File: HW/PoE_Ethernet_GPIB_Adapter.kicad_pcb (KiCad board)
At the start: 6 copper layers, 60 x 55 mm, 198 parts, among them J1 ARJM11C7-114-BA-EW2, J2 112-024-113R001, J3 USB4105-GF-A, J4 UPDI Debug Connector, Q1 PMV30XPEAR, Q2 BC857BS, SW1 Reset, U1 LM5180, U10 AZ1117-3.3_SOT89, U11 TPS2375-1, U2 ATmega4809-A, U3 W5500, U4 24AA256UID, U5 USBLC6-2P6, U6 CH340X, U7 SN74LV1T125DCK, U8 SN74LV1T125DCK, U9 APX811-31UG-7, Y1 25Mhz

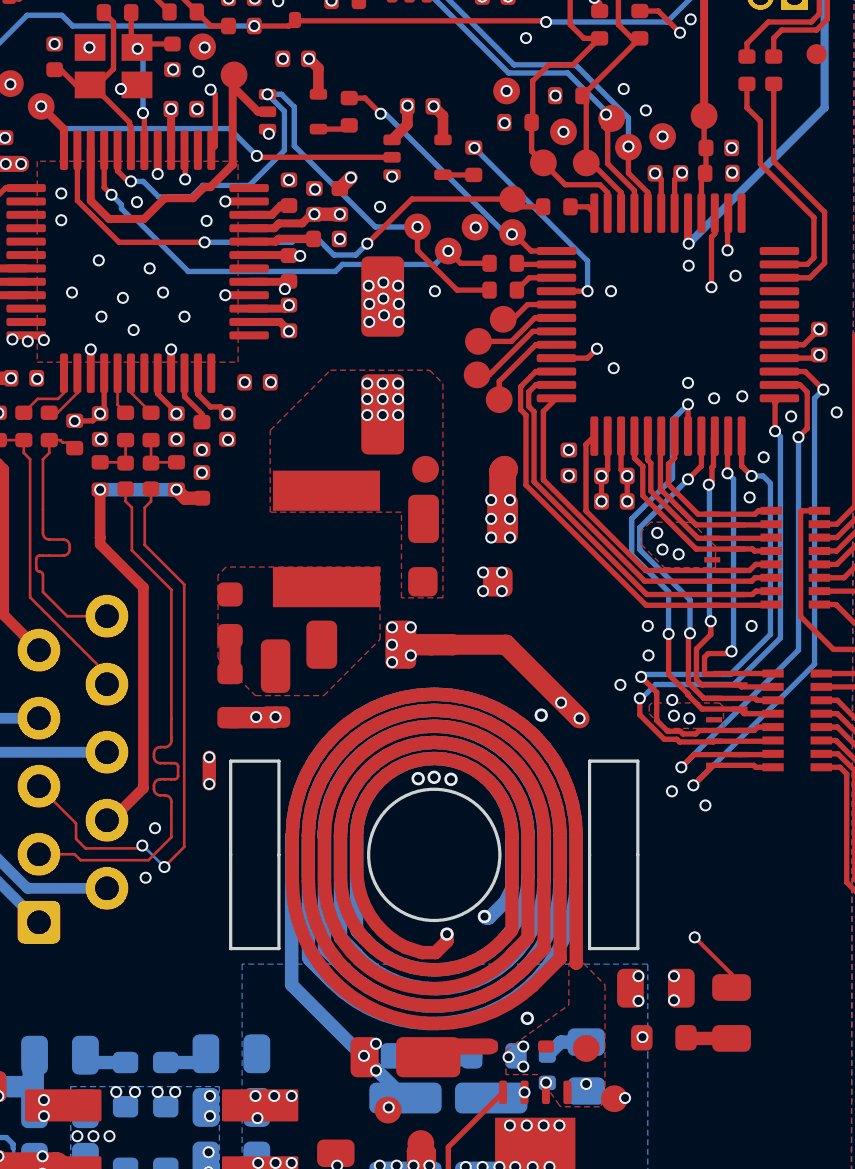
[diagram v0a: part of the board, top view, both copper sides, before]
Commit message: asdf
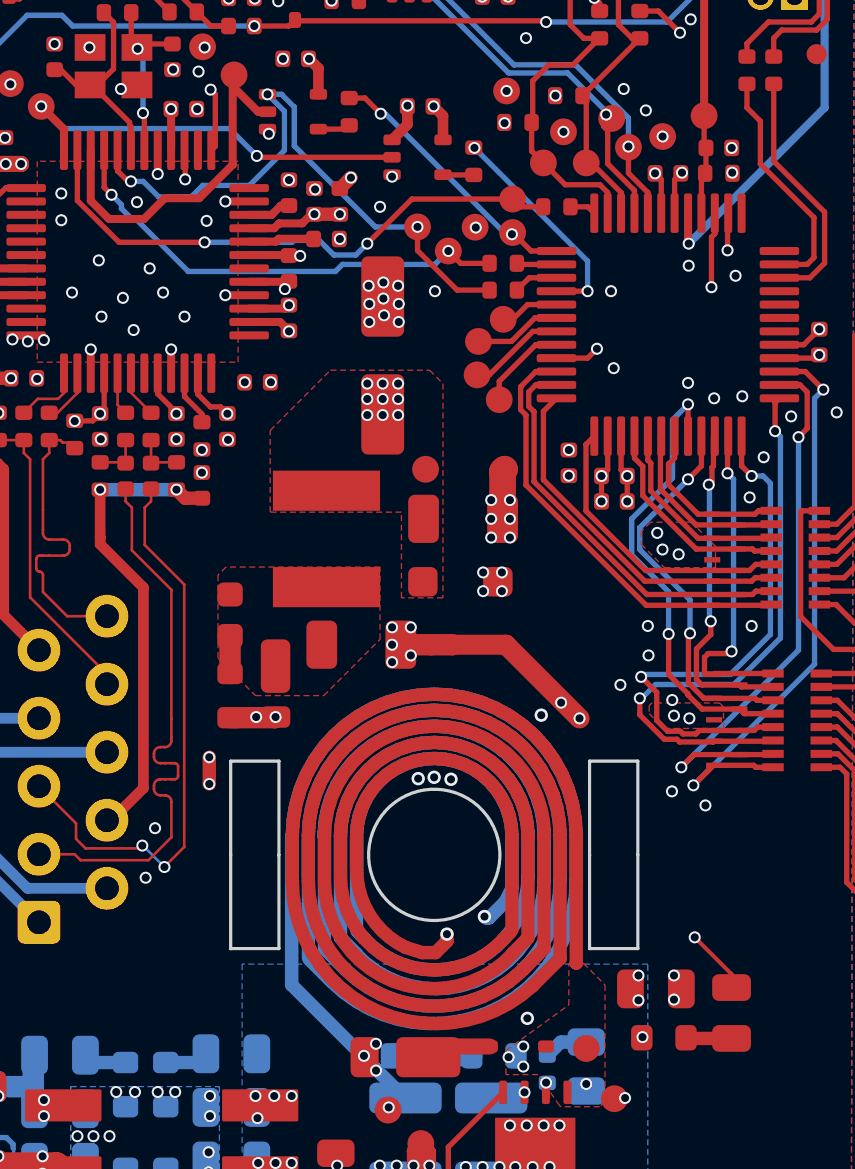
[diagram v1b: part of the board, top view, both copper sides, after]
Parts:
- turned C57 to 180 degrees
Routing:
- net Earth: track 6.68 -> 3.84 mm
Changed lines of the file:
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@@
 	(footprint "Capacitor_SMD:C_0805_2012Metric"
 		(layer "F.Cu")
-		(at 7.4 16.875)
+		(at 7.4 16.9 180)
 		(descr "Capacitor SMD 0805 (2012 Metric), square (rectangular) end terminal, IPC_7351 nominal, (Body size source: IPC-SM-782 page 76, https://www.pcb-3d.com/wordpress/wp-content/uploads/ipc-sm-782a_amendment_1_and_2.pdf, https://docs.google.com/spreadsheets/d/1BsfQQcO9C6DZCsRaXUlFlo91Tg2WpOkGARC1WS5S8t0/edit?usp=sharing), generated with kicad-footprint-generator")
 		(tags "capacitor")
 		(property "Reference" "C57"
-			(at 0 -1.68 0)
+			(at 0 -1.68 360)
 			(layer "User.1")
 			(effects
@@
 		)
 		(property "Value" "4.7n 1kV"
-			(at 0 1.68 0)
+			(at 0 1.68 360)
 			(layer "F.Fab")
 			(effects
@@
 		)
 		(property "Footprint" ""
-			(at 0 0 0)
+			(at 0 0 360)
 			(layer "F.Fab")
 			(hide yes)
@@
 		)
 		(property "Datasheet" ""
-			(at 0 0 0)
+			(at 0 0 180)
 			(unlocked yes)
 			(layer "F.Fab")
@@
 		)
 		(property "Description" "Unpolarized capacitor"
-			(at 0 0 0)
+			(at 0 0 180)
 			(unlocked yes)
 			(layer "F.Fab")
@@
 		)
 		(property "Model" "C0805C472KDRACTU"
-			(at 0 0 0)
+			(at 0 0 180)
 			(unlocked yes)
 			(layer "F.Fab")
@@
 		)
 		(property "Manufacturer" "KEMET"
-			(at 0 0 0)
+			(at 0 0 180)
 			(unlocked yes)
 			(layer "F.Fab")
@@
 		)
 		(property "JLCPCB" "C565695"
-			(at 0 0 0)
+			(at 0 0 180)
 			(unlocked yes)
 			(layer "F.Fab")
@@
 		(attr smd)
 		(fp_line
-			(start -1.7 -0.98)
-			(end 1.7 -0.98)
+			(start 1.7 0.98)
+			(end -1.7 0.98)
 			(stroke
 				(width 0.05)
@@
 		)
 		(fp_line
-			(start -1.7 0.98)
-			(end -1.7 -0.98)
+			(start 1.7 -0.98)
+			(end 1.7 0.98)
 			(stroke
 				(width 0.05)
@@
 		)
 		(fp_line
-			(start 1.7 -0.98)
-			(end 1.7 0.98)
+			(start -1.7 0.98)
+			(end -1.7 -0.98)
 			(stroke
 				(width 0.05)
@@
 		)
 		(fp_line
-			(start 1.7 0.98)
-			(end -1.7 0.98)
+			(start -1.7 -0.98)
+			(end 1.7 -0.98)
 			(stroke
 				(width 0.05)
@@
 		)
 		(fp_line
-			(start -1 -0.625)
-			(end 1 -0.625)
+			(start 1 0.625)
+			(end -1 0.625)
 			(stroke
 				(width 0.1)
@@
 		)
 		(fp_line
-			(start -1 0.625)
-			(end -1 -0.625)
+			(start 1 -0.625)
+			(end 1 0.625)
 			(stroke
 				(width 0.1)
@@
 		)
 		(fp_line
-			(start 1 -0.625)
-			(end 1 0.625)
+			(start -1 0.625)
+			(end -1 -0.625)
 			(stroke
 				(width 0.1)
@@
 		)
 		(fp_line
-			(start 1 0.625)
-			(end -1 0.625)
+			(start -1 -0.625)
+			(end 1 -0.625)
 			(stroke
 				(width 0.1)
@@
 		)
 		(fp_line
-			(start -0.261252 -0.735)
-			(end 0.261252 -0.735)
+			(start -0.261252 0.735)
+			(end 0.261252 0.735)
 			(stroke
 				(width 0.12)
@@
 		)
 		(fp_line
-			(start -0.261252 0.735)
-			(end 0.261252 0.735)
+			(start -0.261252 -0.735)
+			(end 0.261252 -0.735)
 			(stroke
 				(width 0.12)
@@
 		)
 		(fp_text user "${REFERENCE}"
-			(at 0 0 0)
+			(at 0 0 360)
 			(layer "F.Fab")
 			(effects
@@
 		)
 		(pad "1" smd roundrect
-			(at -0.95 0)
+			(at -0.95 0 180)
 			(size 1 1.45)
 			(layers "F.Cu" "F.Mask" "F.Paste")
@@
 		)
 		(pad "2" smd roundrect
-			(at 0.95 0)
+			(at 0.95 0 180)
 			(size 1 1.45)
 			(layers "F.Cu" "F.Mask" "F.Paste")
@@
 					(xy 2.562135 -23.67391) (xy 2.420116 -23.569076) (xy 2.256769 -23.480525) (xy 2.082437 -23.416511)
 					(xy 1.888964 -23.376857) (xy 1.67315 -23.363105) (xy 1.45746 -23.376857) (xy 1.26411 -23.416511)
-					(xy 1.089898 -23.480525) (xy 0.926442 -23.569094) (xy 0.78443 -23.673929) (xy 0.661803 -23.795415)
-					(xy 0.557004 -23.93306) (xy 0.469614 -24.086359) (xy 0.399486 -24.257034) (xy 0.331952 -24.526478)
-					(xy 0.309177 -24.810976) (xy 0.695325 -24.810976) (xy 0.711384 -24.579532) (xy 0.75834 -24.366027)
+					(xy 1.089898 -23.480525) (xy 0.926442 -23.569094) (xy 0.784429 -23.673929) (xy 0.661802 -23.795415)
+					(xy 0.557003 -23.93306) (xy 0.469613 -24.086359) (xy 0.399485 -24.257034) (xy 0.331951 -24.526478)
+					(xy 0.309176 -24.810976) (xy 0.695324 -24.810976) (xy 0.711383 -24.579532) (xy 0.758339 -24.366027)
 					(xy 0.837011 -24.168231) (xy 0.942986 -24.001128) (xy 1.079756 -23.862439) (xy 1.24945 -23.756397)
 					(xy 1.375374 -23.708186) (xy 1.515771 -23.6783) (xy 1.67315 -23.66792) (xy 1.830653 -23.6783) (xy 1.971173 -23.708186)
@@
 					(xy 2.097217 -25.863358) (xy 1.971056 -25.912802) (xy 1.830547 -25.94341) (xy 1.67315 -25.954033)
 					(xy 1.515877 -25.94341) (xy 1.375492 -25.912802) (xy 1.24945 -25.863358) (xy 1.079526 -25.756124)
-					(xy 0.942986 -25.618627) (xy 0.837114 -25.45336) (xy 0.75834 -25.255926) (xy 0.711384 -25.042421)
-					(xy 0.695325 -24.810976) (xy 0.309177 -24.810976) (xy 0.331952 -25.095475) (xy 0.399486 -25.364919)
-					(xy 0.469614 -25.535594) (xy 0.557004 -25.688893) (xy 0.661803 -25.826538) (xy 0.784436 -25.948009)
+					(xy 0.942986 -25.618627) (xy 0.837114 -25.45336) (xy 0.758339 -25.255926) (xy 0.711383 -25.042421)
+					(xy 0.695324 -24.810976) (xy 0.309176 -24.810976) (xy 0.331951 -25.095475) (xy 0.399485 -25.364919)
+					(xy 0.469613 -25.535594) (xy 0.557003 -25.688893) (xy 0.661802 -25.826538) (xy 0.784435 -25.948009)
 					(xy 0.926448 -26.052783) (xy 1.089898 -26.141245) (xy 1.264119 -26.205361) (xy 1.457469 -26.245075)
 					(xy 1.67315 -26.258848)
@@
 				(pts
 					(xy -1.919234 -26.20023) (xy -1.919234 -25.883691) (xy -1.096746 -25.883691) (xy -1.096746 -23.41)
-					(xy -0.710598 -23.41) (xy -0.710598 -25.883691) (xy 0.112073 -25.883691) (xy 0.112073 -26.20023)
+					(xy -0.710598 -23.41) (xy -0.710598 -25.883691) (xy 0.112072 -25.883691) (xy 0.112072 -26.20023)
 				)
 			)
@@
 	)
 	(via
+		(at 8.075 16.4)
+		(size 0.45)
+		(drill 0.3)
+		(layers "F.Cu" "B.Cu")
+		(net 1)
+	)
+	(via
 		(at 5.791994 26.9)
 		(size 0.45)
@@
 	)
 	(via
-		(at 6.75 17.35)
-		(size 0.45)
-		(drill 0.3)
-		(layers "F.Cu" "B.Cu")
-		(net 1)
-	)
-	(via
 		(at 22.4 -27)
 		(size 0.45)
@@
 	)
 	(via
+		(at 8.075 17.3)
+		(size 0.45)
+		(drill 0.3)
+		(layers "F.Cu" "B.Cu")
+		(net 1)
+	)
+	(via
 		(at -2.45 -13.425)
 		(size 0.45)
@@
 	)
 	(via
-		(at 6.75 16.425)
-		(size 0.45)
-		(drill 0.3)
-		(layers "F.Cu" "B.Cu")
-		(net 1)
-	)
-	(via
 		(at 24.929003 26.9)
 		(size 0.45)
@@
 	)
 	(segment
-		(start -13.7 -14.4125)
-		(end -13.7 -12.527979)
-		(width 0.3)
-		(layer "F.Cu")
-		(net 101)
-	)
-	(segment
-		(start -9.47 -13.032979)
-		(end -9.238901 -13.032979)
+		(start -9.65188 -12.62)
+		(end -8.4 -13.87188)
 		(width 0.3)
 		(layer "F.Cu")
@@
 	)
 	(segment
-		(start -13.017021 -11.845)
-		(end -11.714045 -11.845)
-		(width 0.3)
-		(layer "F.Cu")
-		(net 101)
-	)
-	(segment
-		(start -9.882979 -12.62)
-		(end -9.47 -13.032979)
+		(start -10.939045 -12.62)
+		(end -9.65188 -12.62)
 		(width 0.3)
 		(layer "F.Cu")
@@
 	)
 	(segment
-		(start -9.238901 -13.032979)
-		(end -8.4 -13.87188)
+		(start -11.714045 -11.845)
+		(end -10.939045 -12.62)
 		(width 0.3)
 		(layer "F.Cu")
@@
 	)
 	(segment
-		(start -11.714045 -11.845)
-		(end -10.939045 -12.62)
+		(start -13.017021 -11.845)
+		(end -11.714045 -11.845)
 		(width 0.3)
 		(layer "F.Cu")
@@
 	)
 	(segment
-		(start -8.35 -16.75)
-		(end -7.45 -15.85)
+		(start -8.4 -13.87188)
+		(end -8.4 -17.175)
 		(width 0.3)
 		(layer "F.Cu")
@@
 	)
 	(segment
-		(start -8.4 -13.87188)
-		(end -8.4 -17.175)
+		(start -8.35 -16.75)
+		(end -7.45 -15.85)
 		(width 0.3)
 		(layer "F.Cu")
@@
 	)
 	(segment
-		(start -8.35 -17.225)
-		(end -8.35 -16.75)
+		(start -13.7 -12.527979)
+		(end -13.017021 -11.845)
 		(width 0.3)
 		(layer "F.Cu")
@@
 	)
 	(segment
-		(start -13.7 -12.527979)
-		(end -13.017021 -11.845)
+		(start -13.7 -14.4125)
+		(end -13.7 -12.527979)
 		(width 0.3)
 		(layer "F.Cu")
@@
 	)
 	(segment
-		(start -10.939045 -12.62)
-		(end -9.882979 -12.62)
+		(start -8.35 -17.225)
+		(end -8.35 -16.75)
 		(width 0.3)
 		(layer "F.Cu")
@@
 	)
 	(via
-		(at 8.075 16.425)
+		(at 1.95 22)
 		(size 0.45)
 		(drill 0.3)
@@
 	)
 	(via
-		(at 1.95 22)
+		(at 2.8 23.55)
 		(size 0.45)
 		(drill 0.3)
@@
 	)
 	(via
-		(at 2.8 23.55)
+		(at 3.208006 22)
 		(size 0.45)
 		(drill 0.3)
@@
 	)
 	(via
-		(at 3.208006 22)
+		(at 6.75 17.325)
 		(size 0.45)
 		(drill 0.3)
@@
 	)
 	(via
-		(at 8.075 17.325)
-		(size 0.45)
-		(drill 0.3)
-		(layers "F.Cu" "B.Cu")
-		(net 145)
-	)
-	(via
 		(at -0.15 25.2)
 		(size 0.45)
@@
 		(net 145)
 	)
-	(segment
-		(start 7.625 16.425)
-		(end 7.625 17.375)
-		(width 0.5)
-		(layer "In4.Cu")
-		(net 145)
-	)
-	(segment
-		(start 7.625 17.375)
-		(end 7.6 17.4)
-		(width 0.5)
-		(layer "In4.Cu")
-		(net 145)
-	)
-	(segment
-		(start 8.075 16.425)
-		(end 7.625 16.425)
-		(width 0.5)
-		(layer "In4.Cu")
-		(net 145)
-	)
-	(segment
-		(start 8 17.4)
-		(end 8.075 17.325)
-		(width 0.5)
-		(layer "In4.Cu")
-		(net 145)
-	)
-	(segment
-		(start 7.6 17.4)
-		(end 8 17.4)
-		(width 0.5)
-		(layer "In4.Cu")
-		(net 145)
-	)
-	(segment
-		(start 8.075 16.425)
-		(end 8.075 17.325)
-		(width 0.5)
-		(layer "In4.Cu")
+	(via
+		(at 6.75 16.4)
+		(size 0.45)
+		(drill 0.3)
+		(layers "F.Cu" "B.Cu")
 		(net 145)
 	)
